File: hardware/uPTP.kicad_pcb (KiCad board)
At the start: 2 copper layers, 30 x 30 mm, 2 parts, among them U1 CH32V307WCU6, U2 HC-RJ45-055-7

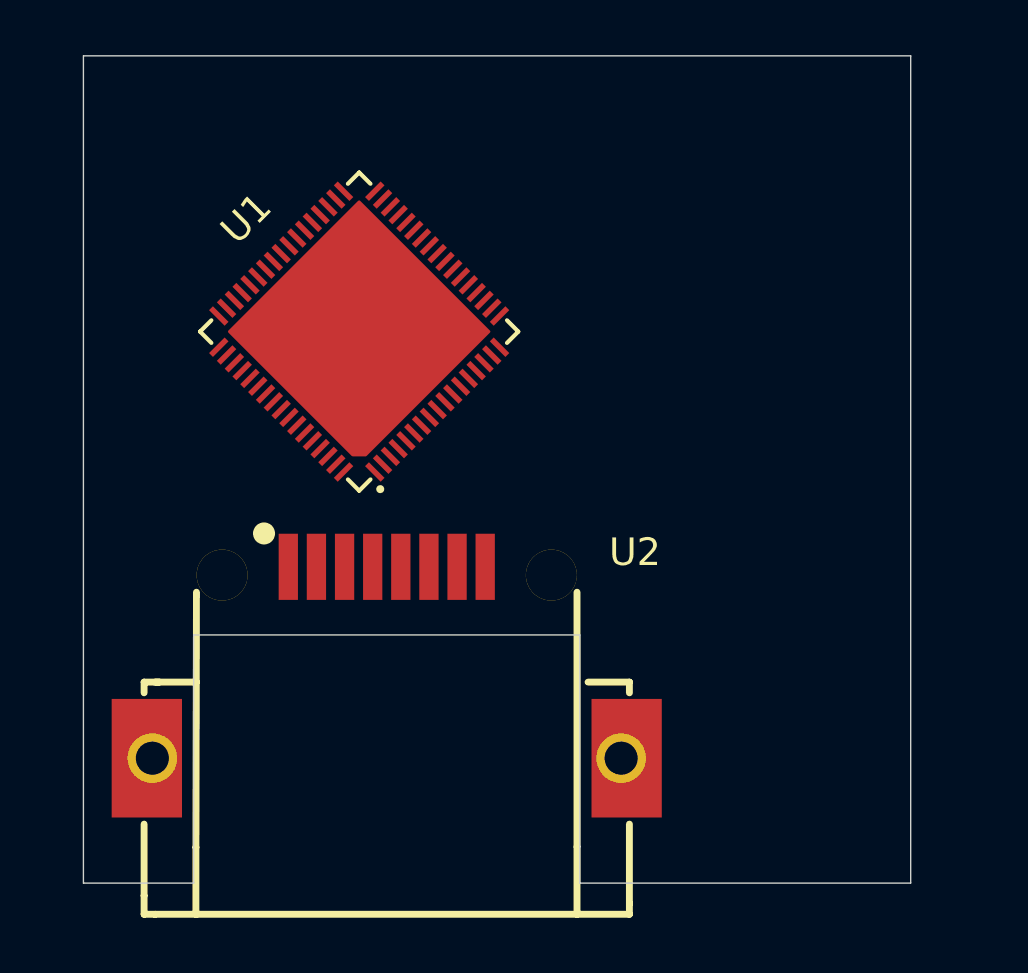
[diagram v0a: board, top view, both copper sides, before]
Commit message: Some more handy components
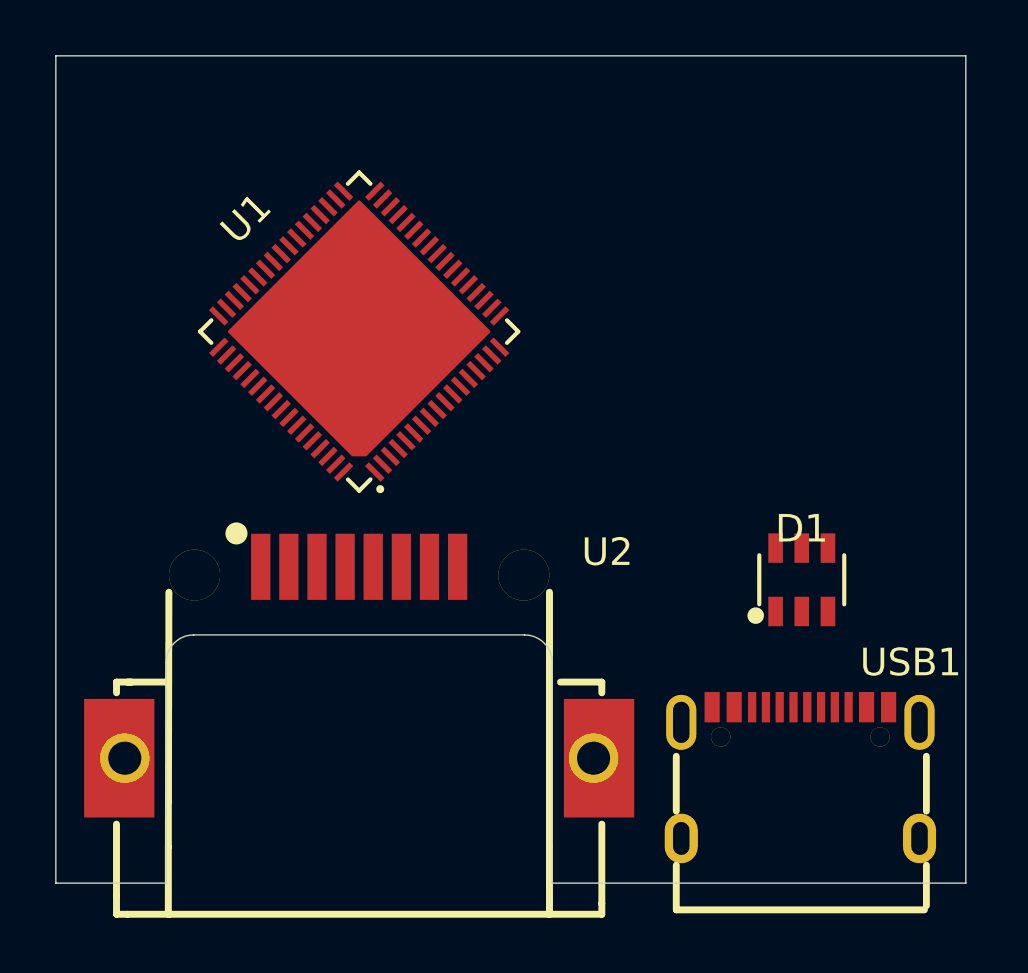
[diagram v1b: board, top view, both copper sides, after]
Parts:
- added D1: USBLC6-2SC6, uPTP:SOT-23-6_L2.9-W1.6-P0.95-LS2.8-BL, F.Cu at (156.1, 119.0)
- added USB1: TYPE-C 16PIN 2MD(073), uPTP:USB-C-SMD_TYPE-C-16PIN, F.Cu at (156.0, 126.0)
- moved U2 1.00 mm to (140.0, 122.0)
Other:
- board size 30 x 30 mm -> 33 x 30 mm
